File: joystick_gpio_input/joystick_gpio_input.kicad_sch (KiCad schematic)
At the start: 27 parts, among them J1 Conn_01x06, J10 Conn_01x14, J11 Conn_01x13, J2 Conn_01x04, J3 Conn_01x15, J4 Conn_01x15, J5 Conn_01x15, J6 Conn_02x09_Odd_Even, J7 Conn_02x09_Odd_Even, J8 Conn_01x14, J9 Conn_01x13

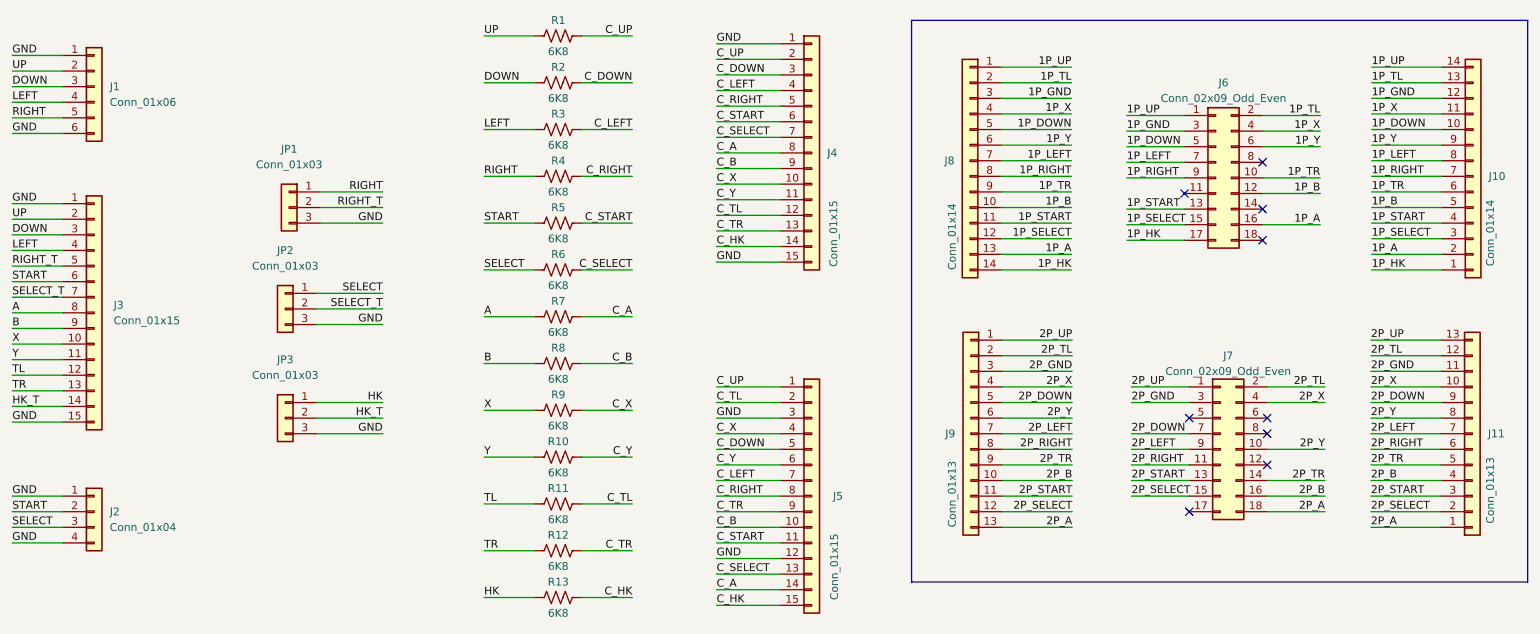
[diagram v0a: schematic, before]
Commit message: Rev 2 설계
Signed-off-by: Ju, Gyeong-min <jcmh74@gmail.com>
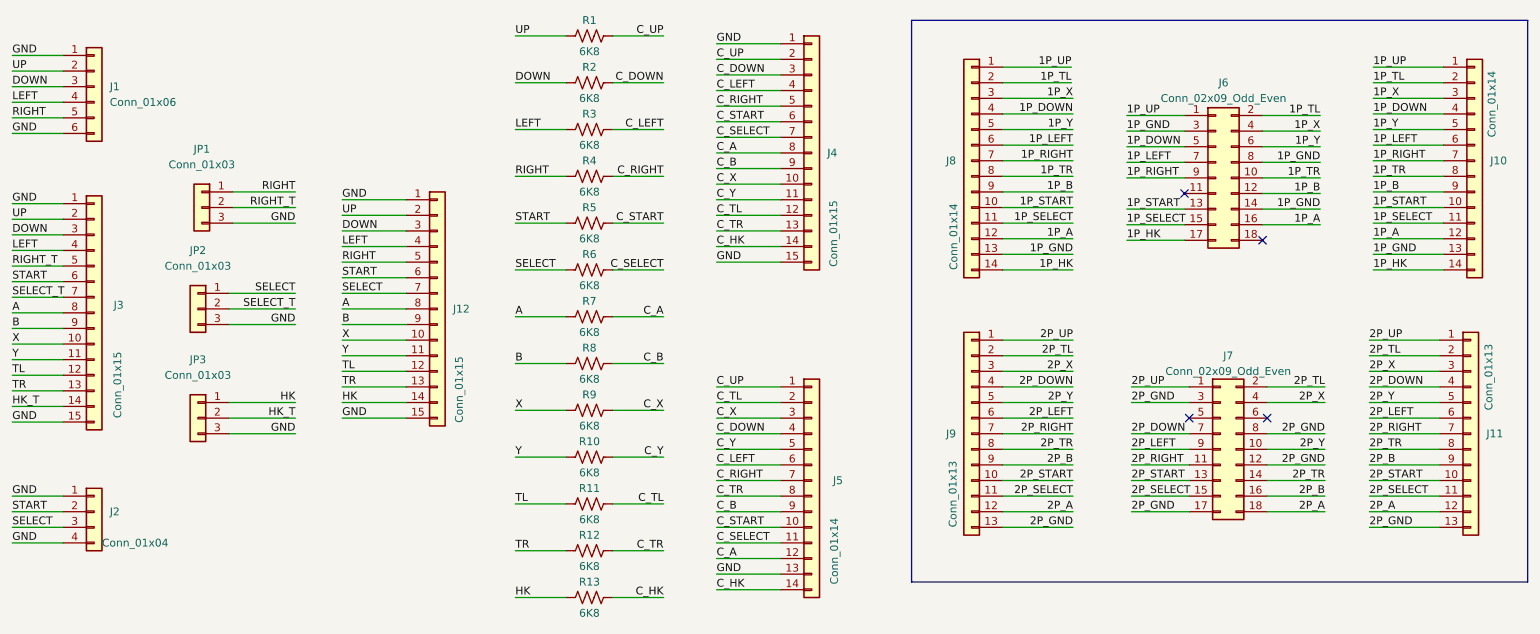
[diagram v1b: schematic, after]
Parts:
- added J12: Conn_01x15, Connector_PinHeader_2.54mm:PinHeader_1x15_P2.54mm_Vertical, symbol Connector_Generic:Conn_01x15
- J10: footprint joystick_gpio_input_library:conn_ex_1x14_P1.25mm_Vertical -> joystick_gpio_input_library:conn_ex_1x14_P1.25mm_Vertical_Left_Labeled
- J11: footprint joystick_gpio_input_library:conn_ex_1x13_P1.25mm_Vertical -> joystick_gpio_input_library:conn_ex_1x13_P1.25mm_Vertical_Left_Labeled
- J5: value Conn_01x15 -> Conn_01x14; footprint Connector_PinHeader_2.54mm:PinHeader_1x15_P2.54mm_Vertical -> joystick_gpio_input_library:conn_ex_1x14_P1.25mm_Vertical_Left_Labeled; symbol Connector_Generic:Conn_01x15 -> Connector_Generic:Conn_01x14
- J8: footprint joystick_gpio_input_library:conn_ex_1x14_P1.25mm_Vertical -> joystick_gpio_input_library:conn_ex_1x14_P1.25mm_Vertical_Right_Labeled
- J9: footprint joystick_gpio_input_library:conn_ex_1x13_P1.25mm_Vertical -> joystick_gpio_input_library:conn_ex_1x13_P1.25mm_Vertical_Right_Labeled
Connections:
- net 1P_A: now also J10.12 (Pin_12), J8.12 (Pin_12); no longer J10.2 (Pin_2), J8.13 (Pin_13)
- net 1P_B: now also J10.9 (Pin_9), J8.9 (Pin_9); no longer J10.5 (Pin_5), J8.10 (Pin_10)
- net 1P_DOWN: now also J10.4 (Pin_4), J8.4 (Pin_4); no longer J10.10 (Pin_10), J8.5 (Pin_5)
- net 1P_GND: now also J10.13 (Pin_13), J6.14 (Pin_14), J6.8 (Pin_8), J8.13 (Pin_13); no longer J10.12 (Pin_12), J8.3 (Pin_3)
- net 1P_HK: now also J10.14 (Pin_14); no longer J10.1 (Pin_1)
- net 1P_LEFT: now also J10.6 (Pin_6), J8.6 (Pin_6); no longer J10.8 (Pin_8), J8.7 (Pin_7)
- net 1P_RIGHT: now also J8.7 (Pin_7); no longer J8.8 (Pin_8)
- net 1P_SELECT: now also J10.11 (Pin_11), J8.11 (Pin_11); no longer J10.3 (Pin_3), J8.12 (Pin_12)
- net 1P_START: now also J10.10 (Pin_10), J8.10 (Pin_10); no longer J10.4 (Pin_4), J8.11 (Pin_11)
- net 1P_TL: now also J10.2 (Pin_2); no longer J10.13 (Pin_13)
- net 1P_TR: now also J10.8 (Pin_8), J8.8 (Pin_8); no longer J10.6 (Pin_6), J8.9 (Pin_9)
- net 1P_UP: now also J10.1 (Pin_1); no longer J10.14 (Pin_14)
- net 1P_X: now also J10.3 (Pin_3), J8.3 (Pin_3); no longer J10.11 (Pin_11), J8.4 (Pin_4)
- net 1P_Y: now also J10.5 (Pin_5), J8.5 (Pin_5); no longer J10.9 (Pin_9), J8.6 (Pin_6)
- net 2P_A: now also J11.12 (Pin_12), J9.12 (Pin_12); no longer J11.1 (Pin_1), J9.13 (Pin_13)
- net 2P_B: now also J11.9 (Pin_9), J9.9 (Pin_9); no longer J11.4 (Pin_4), J9.10 (Pin_10)
- net 2P_DOWN: now also J11.4 (Pin_4), J9.4 (Pin_4); no longer J11.9 (Pin_9), J9.5 (Pin_5)
- net 2P_GND: now also J11.13 (Pin_13), J7.12 (Pin_12), J7.17 (Pin_17), J7.8 (Pin_8), J9.13 (Pin_13); no longer J11.11 (Pin_11), J9.3 (Pin_3)
- net 2P_LEFT: now also J11.6 (Pin_6), J9.6 (Pin_6); no longer J11.7 (Pin_7), J9.7 (Pin_7)
- net 2P_RIGHT: now also J11.7 (Pin_7), J9.7 (Pin_7); no longer J11.6 (Pin_6), J9.8 (Pin_8)
- net 2P_SELECT: now also J11.11 (Pin_11), J9.11 (Pin_11); no longer J11.2 (Pin_2), J9.12 (Pin_12)
- net 2P_START: now also J11.10 (Pin_10), J9.10 (Pin_10); no longer J11.3 (Pin_3), J9.11 (Pin_11)
- net 2P_TL: now also J11.2 (Pin_2); no longer J11.12 (Pin_12)
- net 2P_TR: now also J11.8 (Pin_8), J9.8 (Pin_8); no longer J11.5 (Pin_5), J9.9 (Pin_9)
- net 2P_UP: now also J11.1 (Pin_1); no longer J11.13 (Pin_13)
- net 2P_X: now also J11.3 (Pin_3), J9.3 (Pin_3); no longer J11.10 (Pin_10), J9.4 (Pin_4)
- net 2P_Y: now also J11.5 (Pin_5), J9.5 (Pin_5); no longer J11.8 (Pin_8), J9.6 (Pin_6)
- net A: now also J12.8 (Pin_8)
- net B: now also J12.9 (Pin_9)
- net C_A: now also J5.12 (Pin_12); no longer J5.14 (Pin_14)
- net C_B: now also J5.9 (Pin_9); no longer J5.10 (Pin_10)
- net C_DOWN: now also J5.4 (Pin_4); no longer J5.5 (Pin_5)
- net C_HK: now also J5.14 (Pin_14); no longer J5.15 (Pin_15)
- net C_LEFT: now also J5.6 (Pin_6); no longer J5.7 (Pin_7)
- net C_RIGHT: now also J5.7 (Pin_7); no longer J5.8 (Pin_8)
- net C_SELECT: now also J5.11 (Pin_11); no longer J5.13 (Pin_13)
- net C_START: now also J5.10 (Pin_10); no longer J5.11 (Pin_11)
- net C_TR: now also J5.8 (Pin_8); no longer J5.9 (Pin_9)
- net C_X: now also J5.3 (Pin_3); no longer J5.4 (Pin_4)
- net C_Y: now also J5.5 (Pin_5); no longer J5.6 (Pin_6)
- net DOWN: now also J12.3 (Pin_3)
- net GND: now also J5.13 (Pin_13), J12.1 (Pin_1), J12.15 (Pin_15); no longer J5.12 (Pin_12), J5.3 (Pin_3)
- net HK: now also J12.14 (Pin_14)
- net LEFT: now also J12.4 (Pin_4)
- net RIGHT: now also J12.5 (Pin_5)
- net SELECT: now also J12.7 (Pin_7)
- net START: now also J12.6 (Pin_6)
- net TL: now also J12.12 (Pin_12)
- net TR: now also J12.13 (Pin_13)
- net UP: now also J12.2 (Pin_2)
- net X: now also J12.10 (Pin_10)
- net Y: now also J12.11 (Pin_11)
- no-connect marks 9 -> 4
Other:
- moved on the sheet: JP1, JP2, JP3, R1, R10, R11, R12, R13, R2, R3, R4, R5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
